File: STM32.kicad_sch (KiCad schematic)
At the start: 5 parts

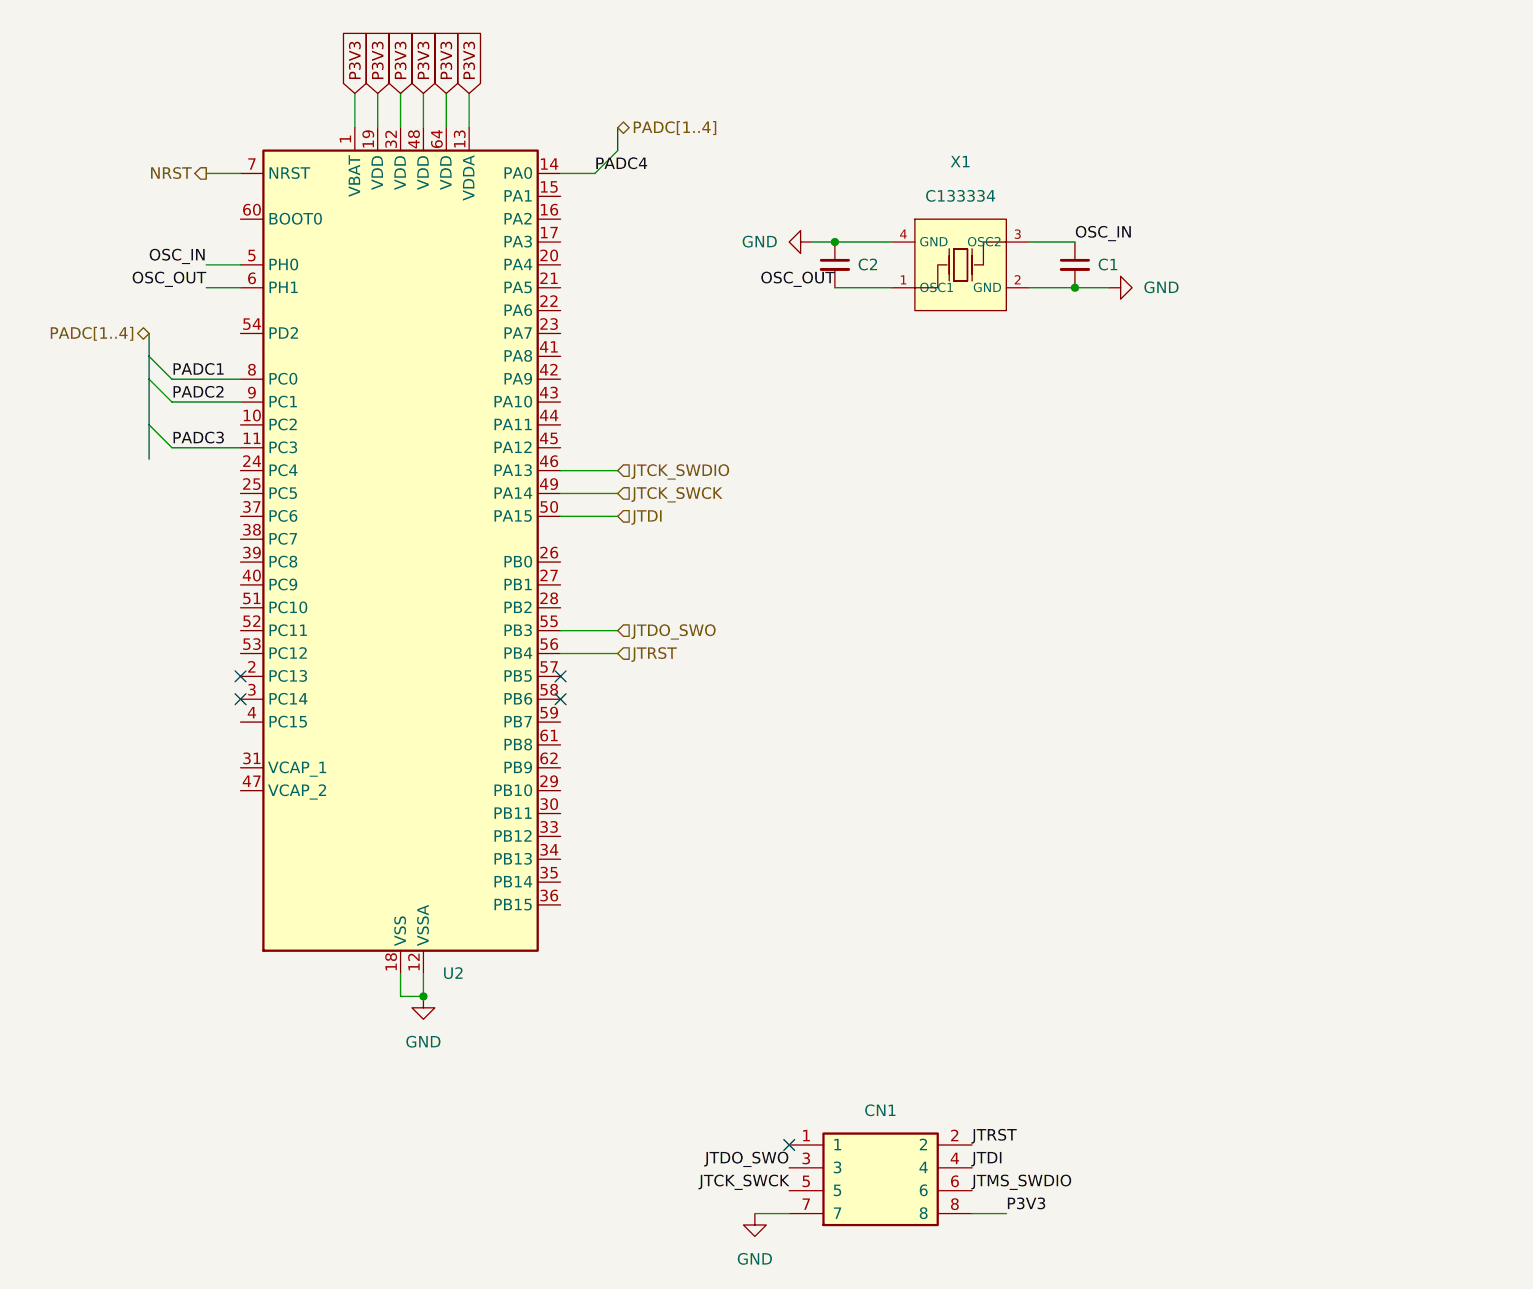
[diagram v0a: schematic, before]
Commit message: 基本完成
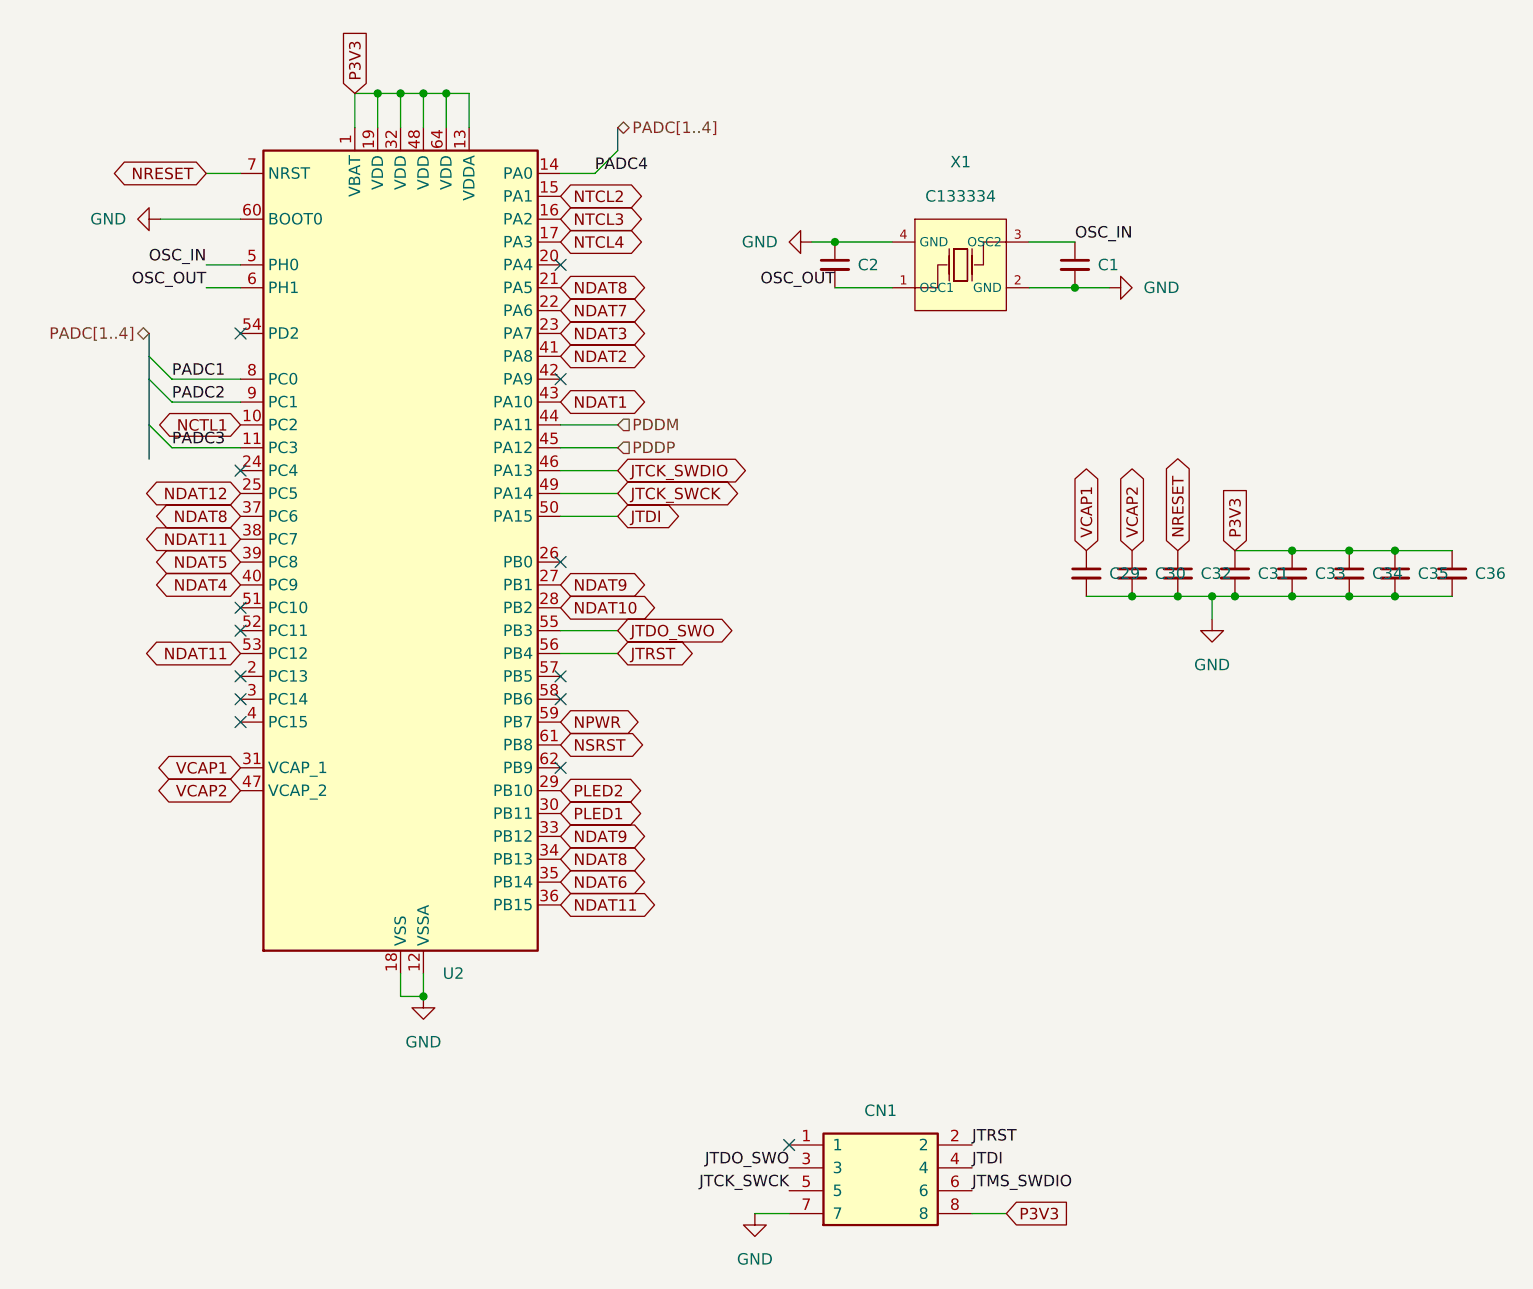
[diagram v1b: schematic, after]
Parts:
- added C29, C30, C31, C32, C33, C34, C35, C36: ~, kicad_community_lib:0603B225K250NT, symbol 0603B225K250NT:0603B225K250NT
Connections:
- net GND: now also U2.60 (BOOT0), C29.2, C30.2, C31.2, C32.2, C33.2, C34.2, C35.2, C36.2
- net P3V3: now also C31.1, C33.1, C34.1, C35.1, C36.1
- net NCTL1: now reaches U2.10 (PC2)
- net NTCL2: now reaches U2.15 (PA1)
- net NTCL3: now reaches U2.16 (PA2)
- net NTCL4: now reaches U2.17 (PA3)
- net NDAT8: now reaches U2.21 (PA5)
- net NDAT8: now also U2.34 (PB13), U2.37 (PC6)
- net NDAT7: now reaches U2.22 (PA6)
- net NDAT3: now reaches U2.23 (PA7)
- net NDAT12: now reaches U2.25 (PC5)
- net NDAT9: now reaches U2.27 (PB1)
- net NDAT9: now also U2.33 (PB12)
- net NDAT10: now reaches U2.28 (PB2)
- net PLED2: now reaches U2.29 (PB10)
- net PLED1: now reaches U2.30 (PB11)
- net VCAP1: now reaches U2.31 (VCAP_1)
- net VCAP1: now also C29.1
- net NDAT6: now reaches U2.35 (PB14)
- net NDAT11: now reaches U2.36 (PB15)
- net NDAT11: now also U2.38 (PC7), U2.53 (PC12)
- net NDAT5: now reaches U2.39 (PC8)
- net NDAT4: now reaches U2.40 (PC9)
- net NDAT2: now reaches U2.41 (PA8)
- net NDAT1: now reaches U2.43 (PA10)
- net PDDM: now reaches U2.44 (PA11)
- net PDDP: now reaches U2.45 (PA12)
- net VCAP2: now reaches U2.47 (VCAP_2)
- net VCAP2: now also C30.1
- net NPWR: now reaches U2.59 (PB7)
- net NSRST: now reaches U2.61 (PB8)
- net NRST renamed NRESET
- net NRESET: now also C32.1
- no-connect marks 5 -> 14
